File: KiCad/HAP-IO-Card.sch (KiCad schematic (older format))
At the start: 0 parts

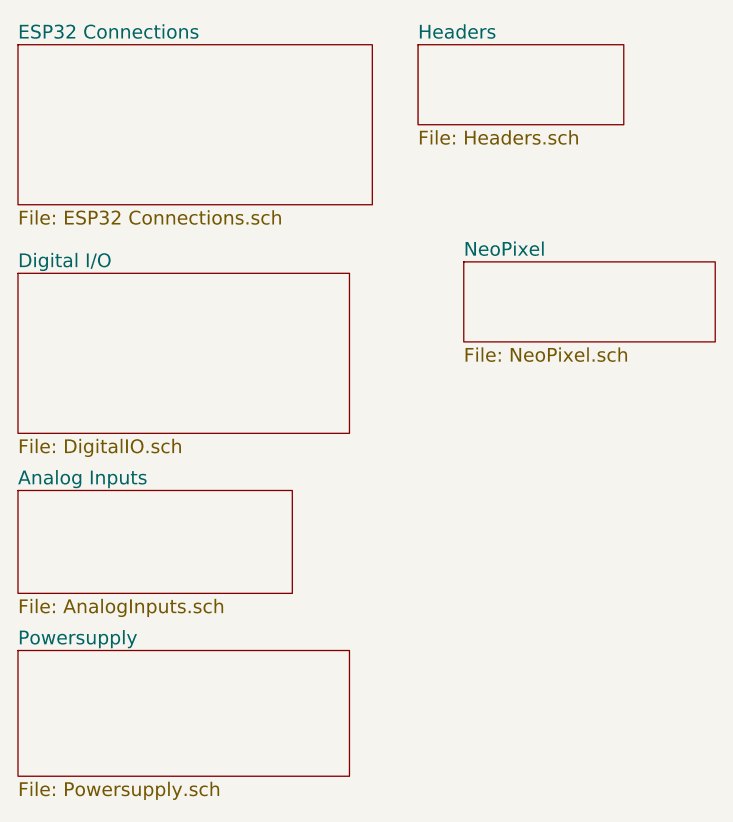
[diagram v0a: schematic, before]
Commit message: More work
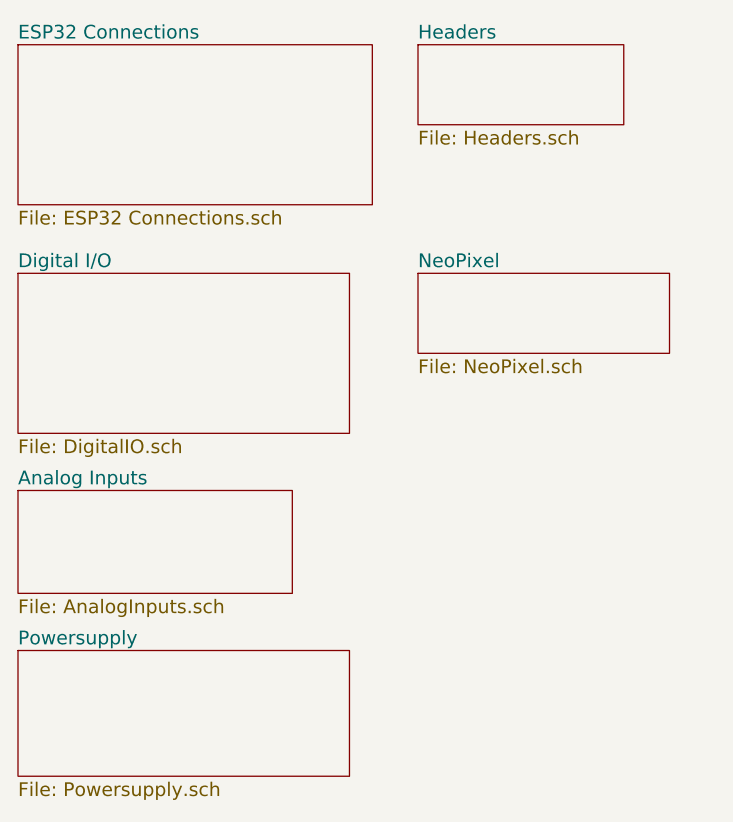
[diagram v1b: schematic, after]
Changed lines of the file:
@@
 EESchema Schematic File Version 2
-LIBS:HAP-IO-Card-rescue
 LIBS:power
 LIBS:device
@@
 $EndSheet
 $Sheet
-S 2850 1750 1100 350
+S 2650 1800 1100 350
 U 5924F41E
 F0 "NeoPixel" 60
